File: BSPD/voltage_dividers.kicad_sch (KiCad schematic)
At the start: 5 parts

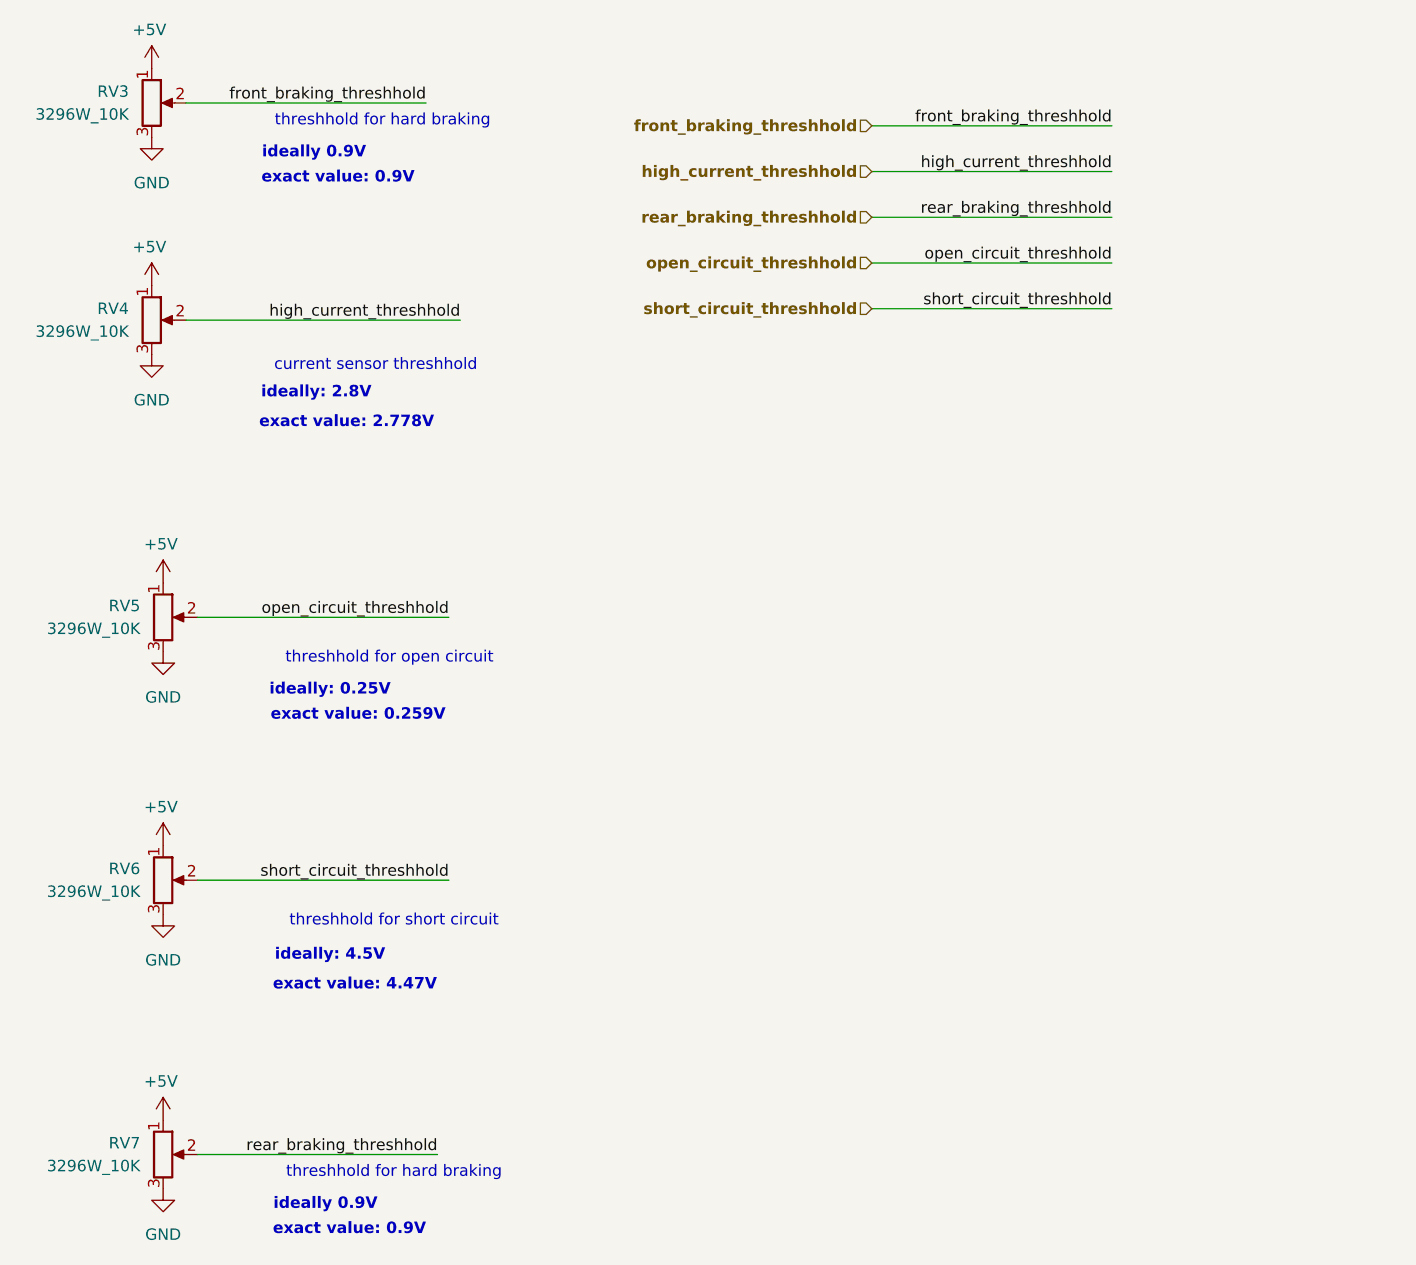
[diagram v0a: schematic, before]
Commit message: all BSPD changes
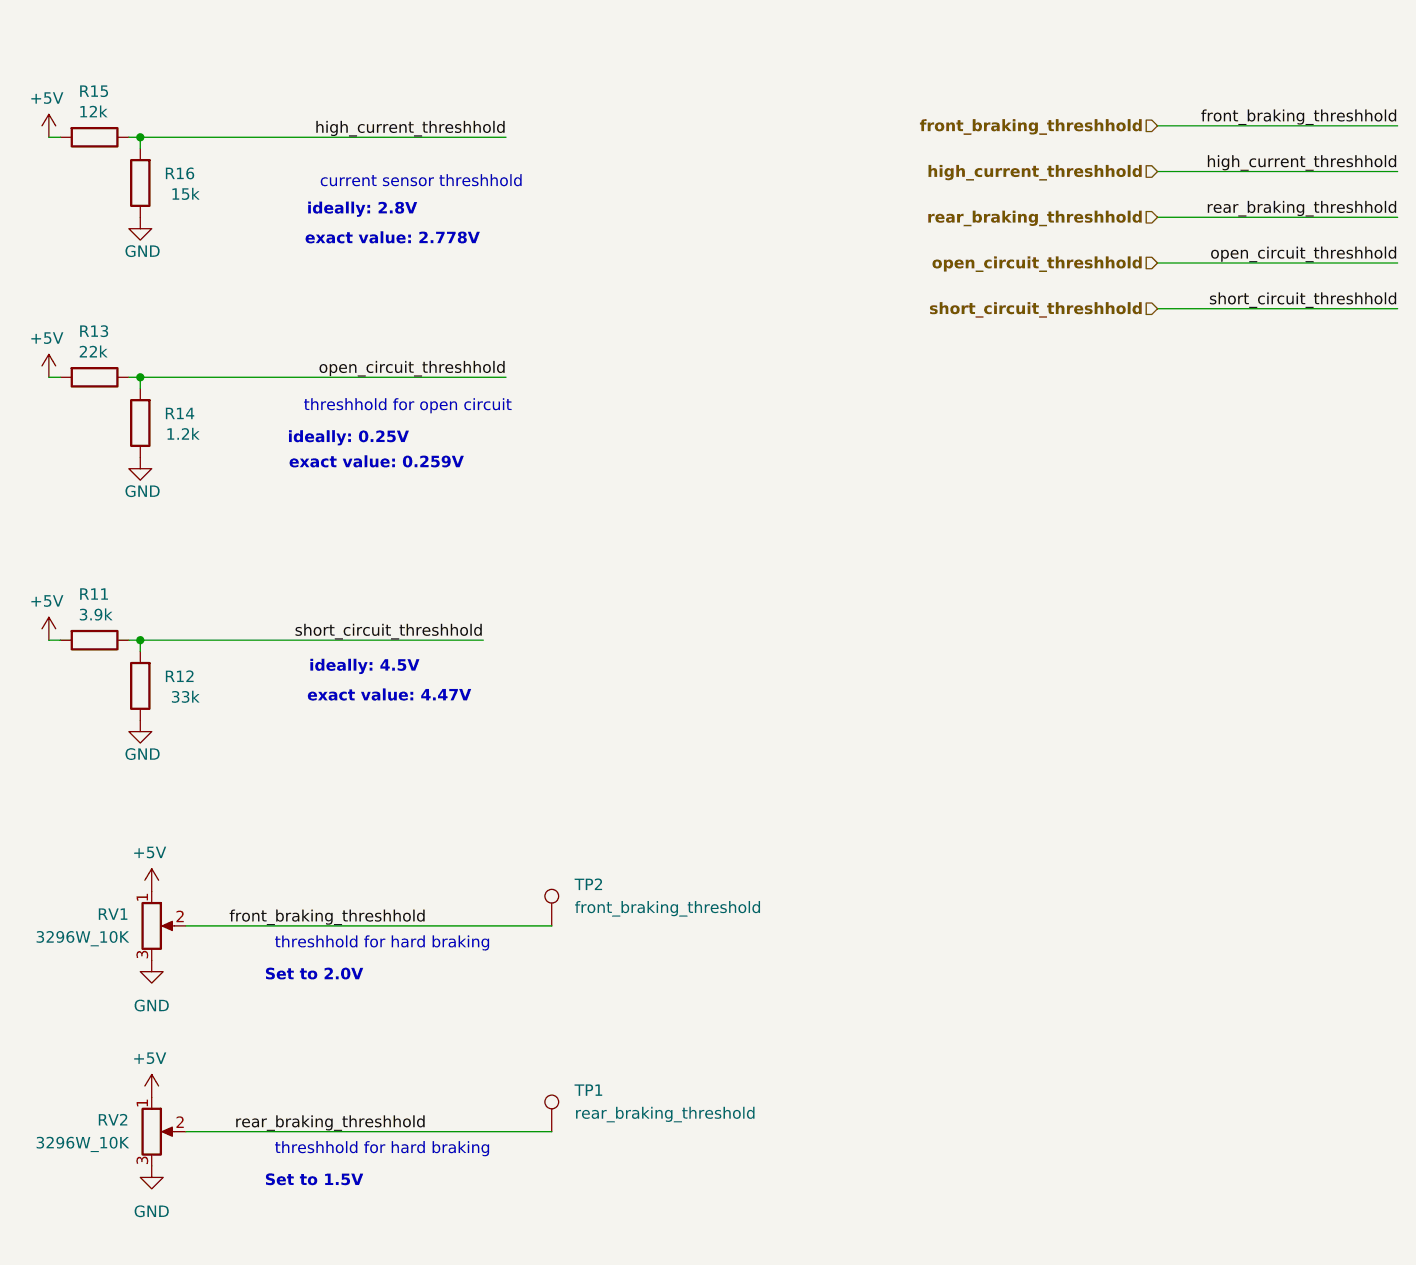
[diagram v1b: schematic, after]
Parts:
- removed RV4, RV5, RV6: 3296W_10K, Potentiometer_THT:Potentiometer_Bourns_3296W_Vertical, symbol Device:R_Potentiometer
- added R11: 3.9k, Resistor_SMD:R_0805_2012Metric_Pad1.20x1.40mm_HandSolder, symbol Device:R
- added R12: 33k, Resistor_SMD:R_0805_2012Metric_Pad1.20x1.40mm_HandSolder, symbol Device:R
- added R13: 22k, Resistor_SMD:R_0805_2012Metric_Pad1.20x1.40mm_HandSolder, symbol Device:R
- added R14: 1.2k, Resistor_SMD:R_0805_2012Metric_Pad1.20x1.40mm_HandSolder, symbol Device:R
- added R15: 12k, Resistor_SMD:R_0805_2012Metric_Pad1.20x1.40mm_HandSolder, symbol Device:R
- added R16: 15k, Resistor_SMD:R_0805_2012Metric_Pad1.20x1.40mm_HandSolder, symbol Device:R
- added TP1: rear_braking_threshold, Connector_PinHeader_2.54mm:PinHeader_1x01_P2.54mm_Vertical, symbol Connector:TestPoint
- added TP2: front_braking_threshold, Connector_PinHeader_2.54mm:PinHeader_1x01_P2.54mm_Vertical, symbol Connector:TestPoint
- renumbered RV3 to RV1, RV7 to RV2
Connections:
- net +5V: now also R11.2, R13.2, R15.2
- net GND: now also R12.1, R14.1, R16.1
- net front_braking_threshhold: now also TP2.1
- net high_current_threshhold: now also R15.1, R16.2
- net open_circuit_threshhold: now also R13.1, R14.2
- net rear_braking_threshhold: now also TP1.1
- net short_circuit_threshhold: now also R11.1, R12.2
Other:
- note added: "Set to 1.5V"
- note added: "Set to 2.0V"
- note removed: "exact value: 0.9V"
- note removed: "ideally 0.9V"
- note removed: "threshhold for short circuit"
- moved on the sheet: RV1, RV2
